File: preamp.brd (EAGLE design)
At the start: 100 x 92.7 mm, 73 parts, among them IC1 INA217DW, IC2 OPA134U, IC3 PCM1808, IC4 12.288MHz, IC5 REG1117

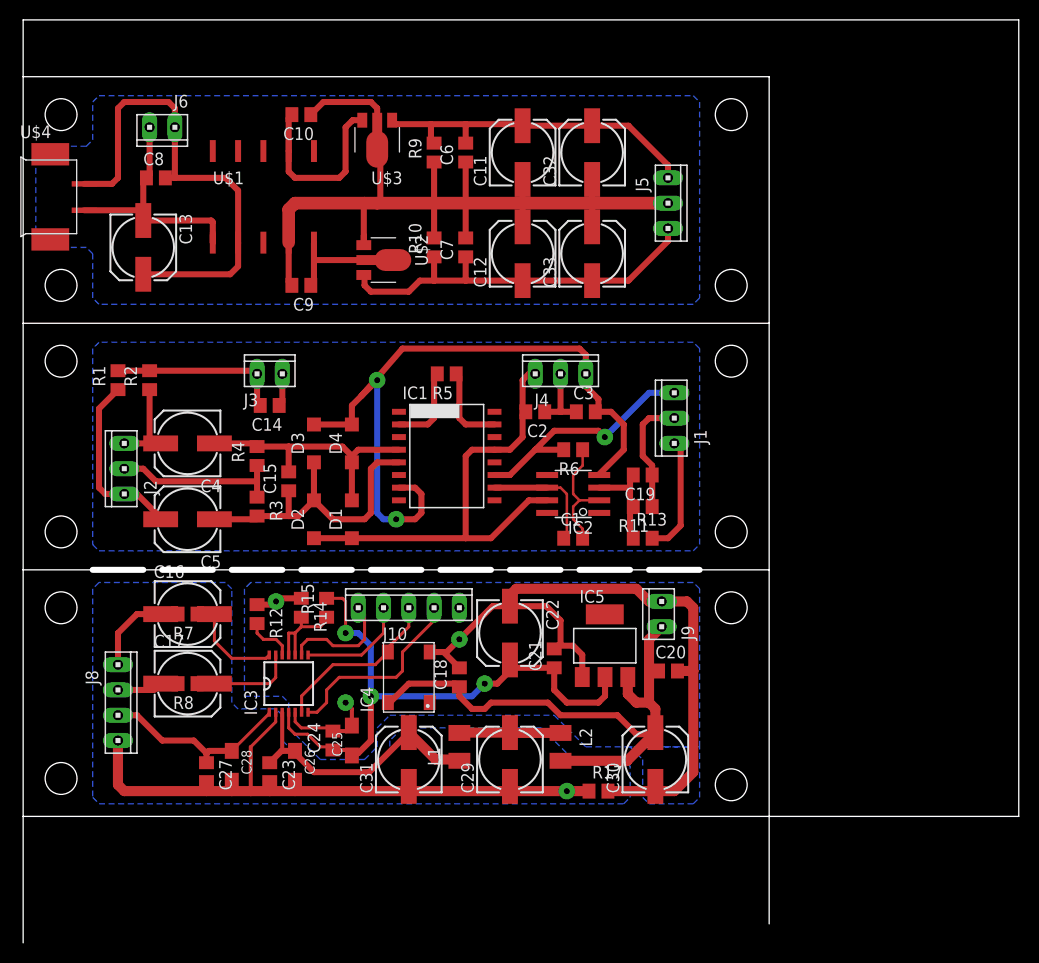
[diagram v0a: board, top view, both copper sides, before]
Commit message: first production
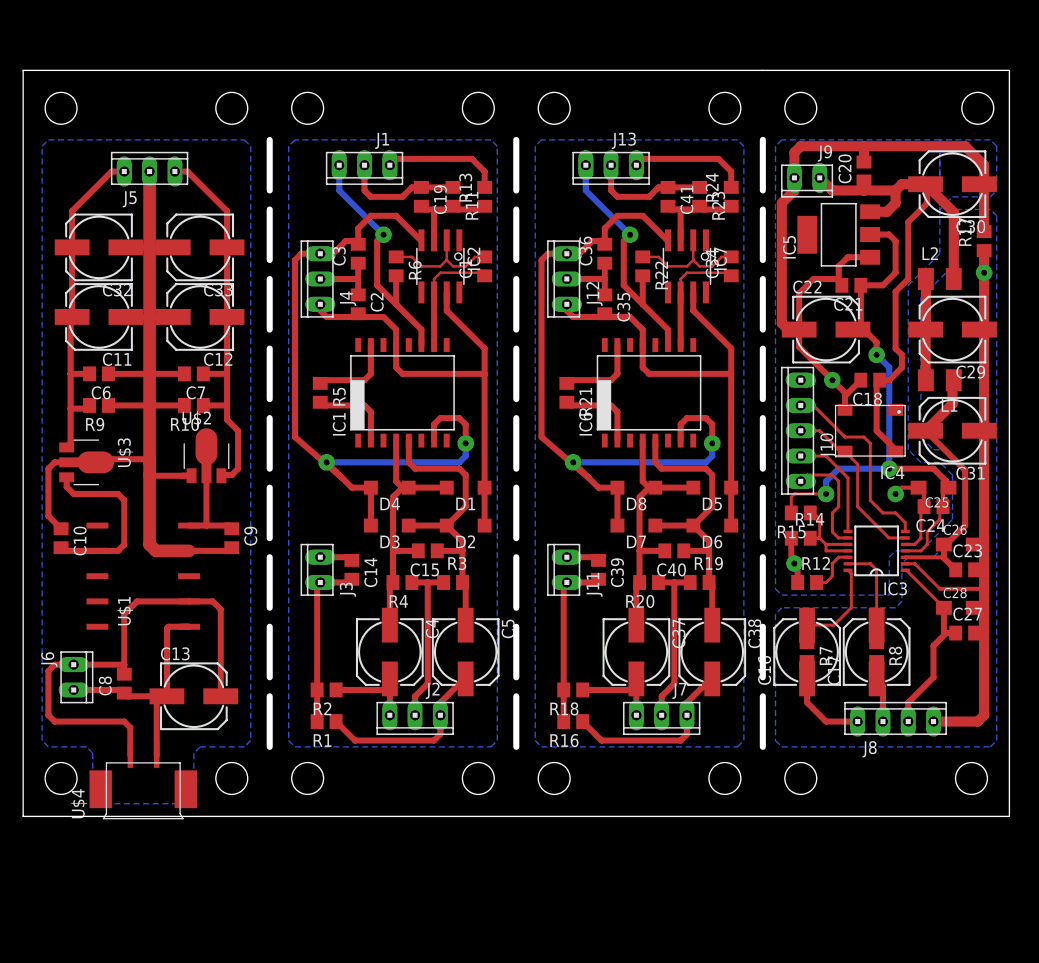
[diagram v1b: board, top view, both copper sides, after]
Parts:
- added C34, C35, C36, C39, C41: 0.1, rcl:C0805
- added C37, C38: 47, rcl:153CLV-0605
- added C40: 470pf, rcl:C0805
- added D5, D6, D7, D8: (no value), diode:SOD123
- added IC6: INA217DW, burr-brown:DW_RPDSO-G16
- added IC7: OPA134U, burr-brown:SO08
- added J11: (no value), con-amp:10X02MTA
- added J12, J13, J7: (no value), con-amp:10X03MTA
- added R16, R18: 1.2k, rcl:R0805
- added R19, R20: 2.2k, rcl:R0805
- added R21: (no value), rcl:R0805
- added R22: 1M, rcl:R0805
- added R23, R24: 0, rcl:R0805
- moved J8 78.1 mm to (87.6, 9.53), turned to 0 degrees
- moved C27 77.5 mm to (94.6, 18.4), turned to 0 degrees
- moved C28 74.7 mm to (94.0, 21.0), turned to 0 degrees
- moved C23 72.7 mm to (94.6, 24.8), turned to 0 degrees
- moved C26 70.3 mm to (94.0, 27.3), turned to 0 degrees
- moved C17 69.3 mm to (85.7, 16.5), turned to 90 degrees
- moved R8 69.3 mm to (85.7, 16.5), turned to 270 degrees
- moved R17 67.5 mm to (96.5, 57.8), turned to 90 degrees
- moved C30 65.0 mm to (93.3, 63.5), turned to 180 degrees
- moved C24 64.7 mm to (91.4, 31.1), turned to 180 degrees
- moved C31 63.8 mm to (93.3, 38.7), turned to 180 degrees
- moved C25 63.7 mm to (91.4, 33.0), turned to 180 degrees
- moved C16 62.3 mm to (78.7, 16.5), turned to 90 degrees
- moved R7 62.3 mm to (78.7, 16.5), turned to 270 degrees
- moved C29 62.0 mm to (93.3, 48.9), turned to 180 degrees
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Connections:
- new net AGND1: C35.1, C36.1, C39.1, C41.1, J11.1, J12.2, J13.2, J7.2, R19.1, R20.1, R23.1
- new net N$29: IC6.2, R21.2
- new net N$30: IC6.15, R21.1
- new net N$31: C38.-, C40.1, D6.A, D7.C, IC6.5, R19.2
- new net N$32: C37.+, J7.1, R18.1
- new net N$33: C38.+, J7.3, R16.1
- new net N$34: C37.-, C40.2, D5.A, D8.C, IC6.4, R20.2
- new net N$35: C39.2, J11.2, R16.2, R18.2
- new net N$36: C34.2, IC7.2, R22.1
- new net N$37: IC6.11, J13.1, R22.2
- new net N$38: C34.1, IC6.10, IC7.6
- new net N$39: C41.2, IC7.3, R23.2, R24.1
- new net N$40: J13.3, R24.2
- new net V+1: C35.2, D5.C, D6.C, IC6.13, IC7.7, J12.3
- new net V-1: C36.2, D7.A, D8.A, IC6.7, IC7.4, J12.1
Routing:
- net V-1: track 0.00 -> 72.9 mm, vias 0 -> 2
- net V+1: track 0.00 -> 47.7 mm
- net AGND1: track 0.00 -> 39.4 mm
- net N$31: track 0.00 -> 31.6 mm
- net N$34: track 0.00 -> 26.5 mm
- net N$37: track 0.00 -> 24.9 mm, vias 0 -> 1
- net N$33: track 0.00 -> 18.2 mm
- net N$35: track 0.00 -> 17.4 mm
- net N$38: track 0.00 -> 12.6 mm
- net N$36: track 0.00 -> 12.2 mm
- net N$40: track 0.00 -> 11.9 mm
- net N$39: track 0.00 -> 9.98 mm
- net N$32: track 0.00 -> 9.05 mm
- net N$29: track 0.00 -> 8.37 mm
- net N$30: track 0.00 -> 8.37 mm
- added copper zone on layer 16, net AGND1
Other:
- board size 100 x 92.7 mm -> 99.1 x 74.9 mm
